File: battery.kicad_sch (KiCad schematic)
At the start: 105 parts, among them J10 SOLAR, J9 Conn_01x02, Q10 SI2308, Q11 CSD17581Q3A, Q5 AON7534, Q6 AON7534, Q7 CSD18512Q5B, Q8 CSD18512Q5B, Q9 SI2308, SW3 POWER/RESET, U7 MAX17320G22+, U8 BQ25798

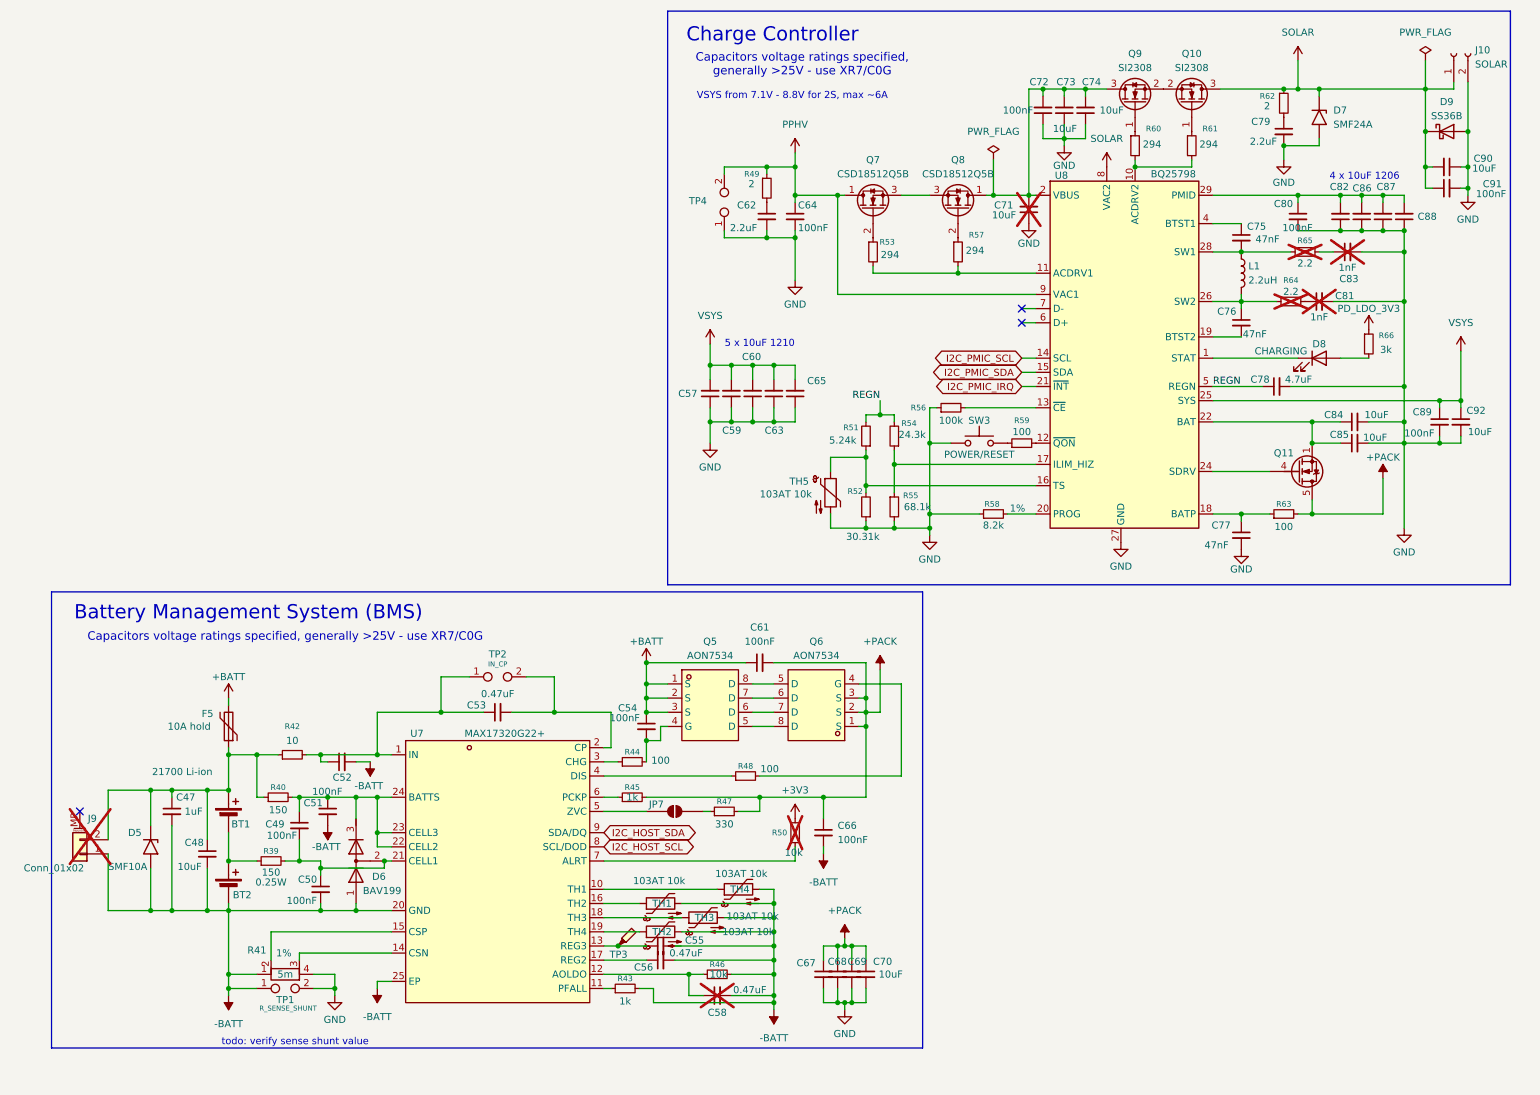
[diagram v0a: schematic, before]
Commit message: organize repo and schematic
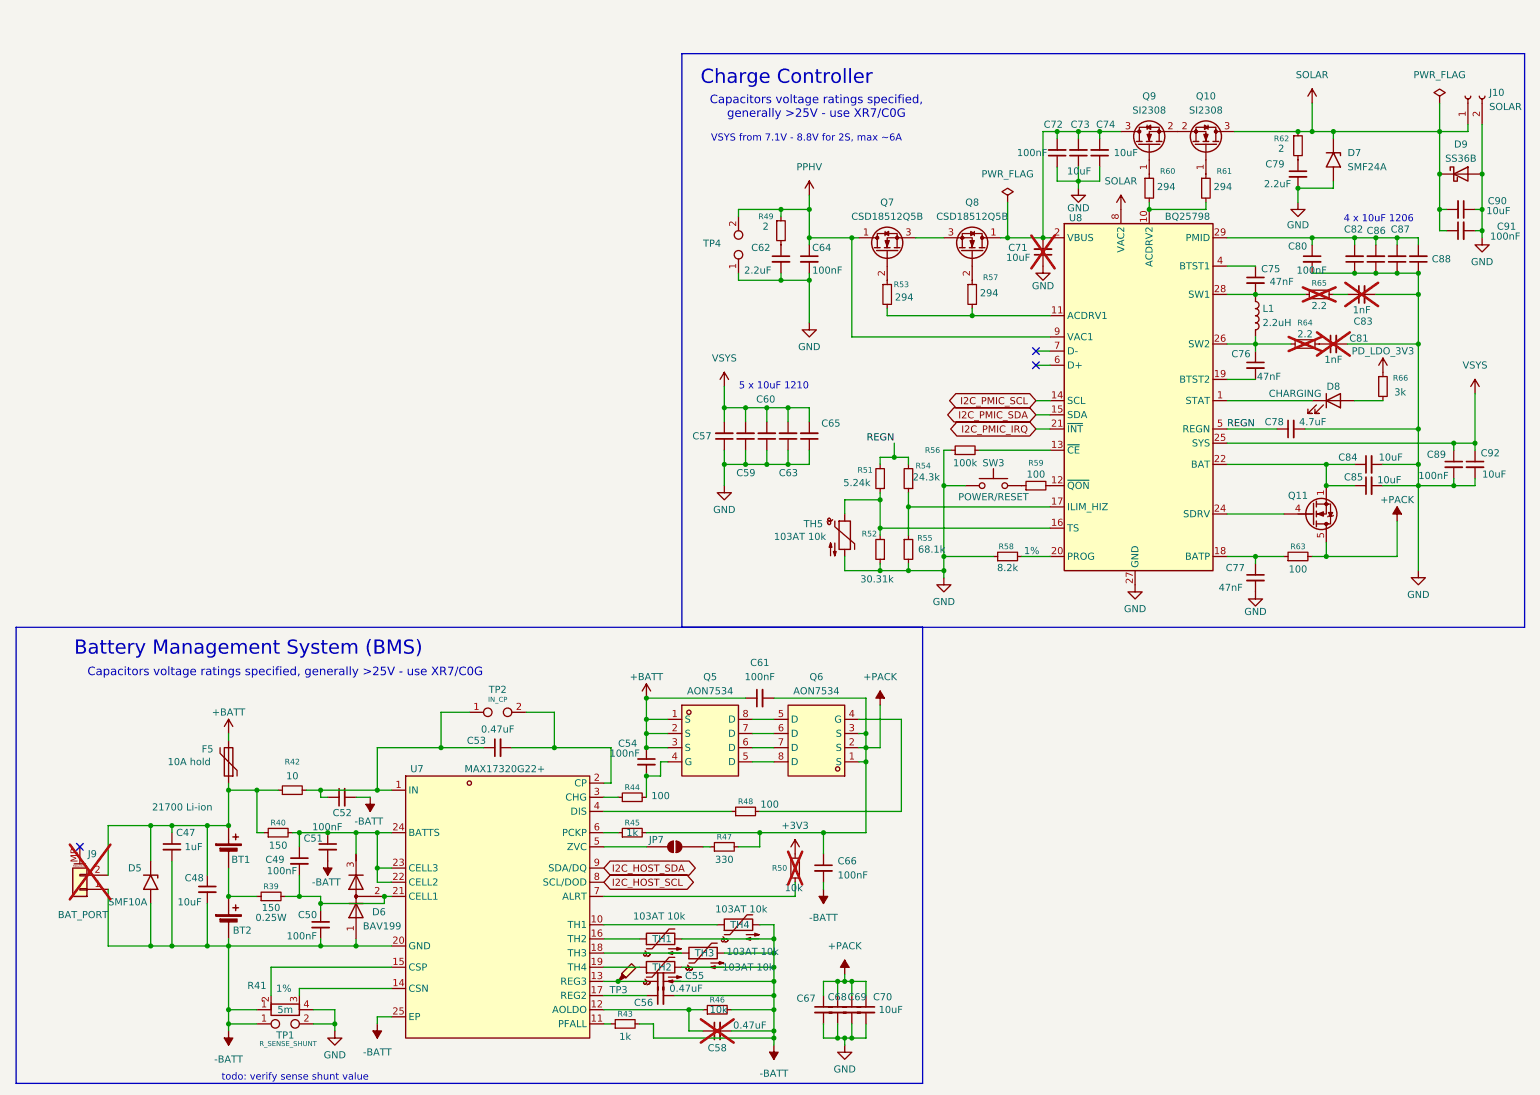
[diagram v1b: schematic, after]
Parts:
- J9: value Conn_01x02 -> BAT_PORT
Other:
- moved on the sheet: BT1, BT2, C47, C48, C49, C50, C51, C52, C53, C54, C55, C56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
